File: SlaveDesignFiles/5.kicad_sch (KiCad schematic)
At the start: 43 parts, among them Q1 TXB0104PWR, Q2 TPS27082LDDCR, Q3 TPT75176B-SO1R, Q4 TPT75176B-SO1R

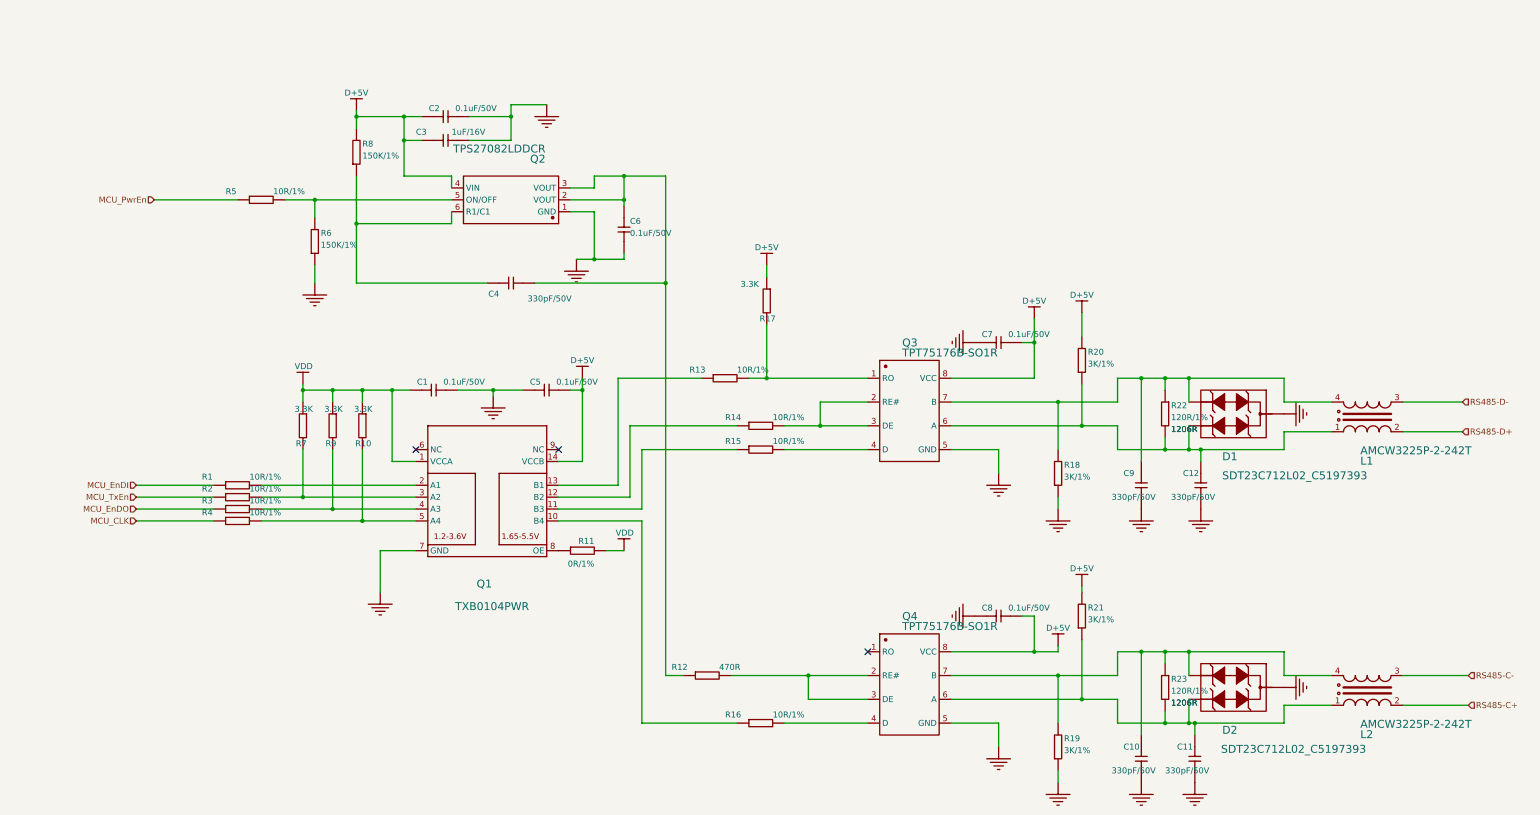
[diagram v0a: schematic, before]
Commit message: 28388d直接在底板上
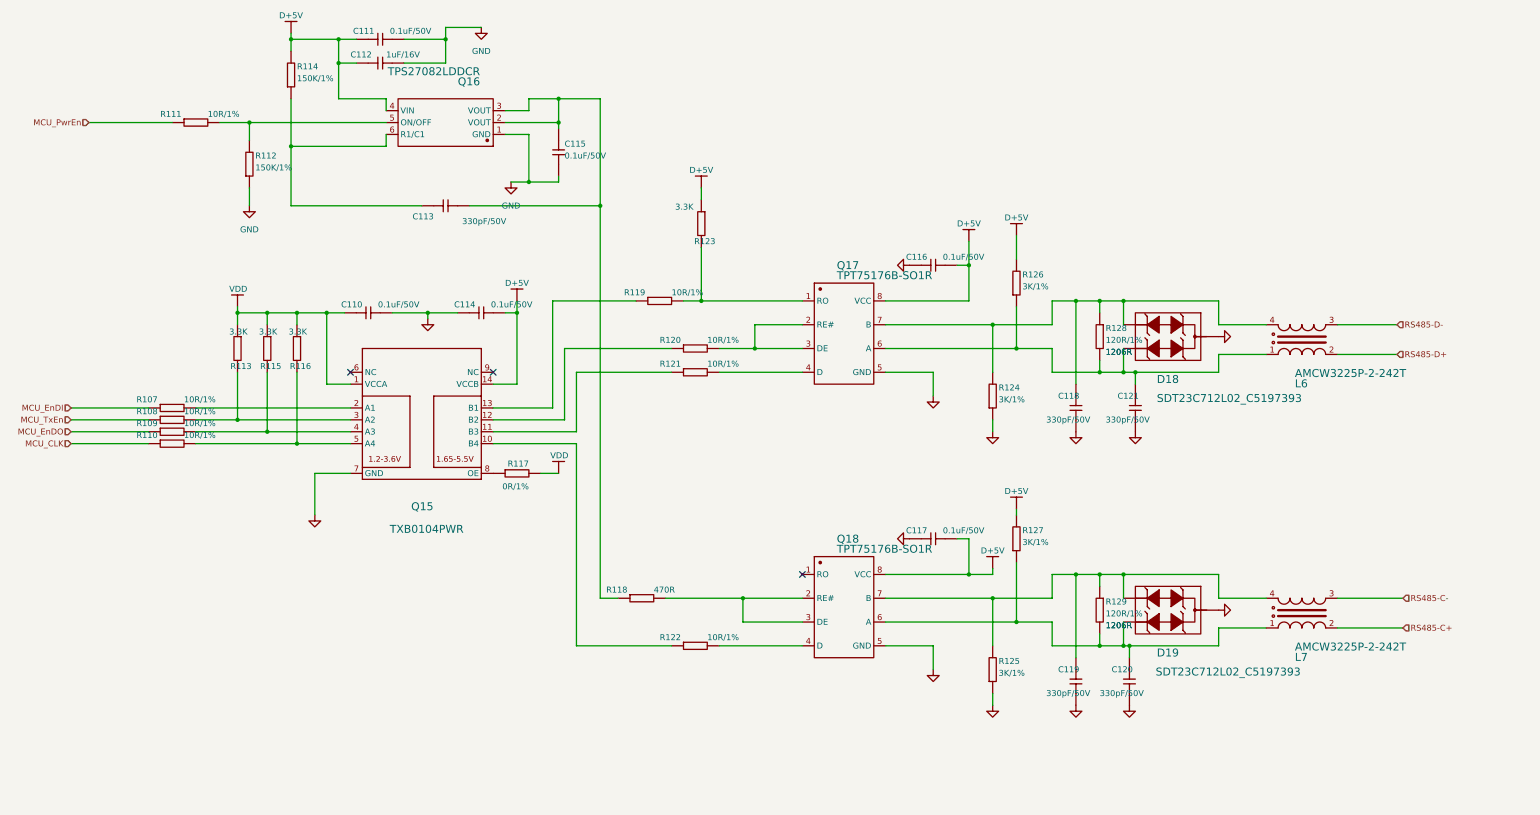
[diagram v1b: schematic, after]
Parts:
- removed C1, C2, C5, C6, C7, C8: 0.1uF/50V, Capacitor_SMD:C_0603_1608Metric, symbol sheet1-altium-import:CAP_2
- removed C10, C11, C12, C4, C9: 330pF/50V, Capacitor_SMD:C_0603_1608Metric, symbol sheet1-altium-import:CAP_1
- removed C3: 1uF/16V, Capacitor_SMD:C_0603_1608Metric, symbol sheet1-altium-import:CAP
- removed D1, D2: SDT23C712L02_C5197393, Lib2ic:SOT-23-3_L2.9-W1.3-P1.90-LS2.4-BR, symbol sheet1-altium-import:SDT23C712L02_C5197393
- removed L1, L2: AMCW3225P-2-242T, Lib_sheet_10:FILTER-SMD_4P-L3.2-W2.5-BL_WCM3225XXXX, symbol sheet1-altium-import:AMCW3225P-2-242T
- removed Q1: TXB0104PWR, Lib2ic:TSSOP-14_L5.0-W4.4-P0.65-LS6.4-BL, symbol sheet1-altium-import:TXB0104PWR
- removed Q2: TPS27082LDDCR, Lib_sheet_10:SOT-23-6_L2.9-W1.6-P0.95-LS2.8-BR, symbol sheet1-altium-import:TPS27082LDDCR
- removed Q3: TPT75176B-SO1R, Lib2ic:SOP-8_L4.9-W3.9-P1.27-LS6.0-BL, symbol sheet1-altium-import:TPT75176B-SO1R
- removed R1, R13, R14, R15, R16, R2, R3, R4, R5: 10R/1%, Resistor_SMD:R_0603_1608Metric, symbol sheet1-altium-import:RES_1
- removed R10, R17, R7, R9: 3.3K, Lib_sheet_10:R_0603_1608Metric, symbol sheet1-altium-import:RES_2
- removed R11: 0R/1%, Resistor_SMD:R_0603_1608Metric, symbol sheet1-altium-import:RES_7
- removed R12: 470R, Resistor_SMD:R_0603_1608Metric, symbol sheet1-altium-import:RES_6
- removed R18, R19, R20, R21: 3K/1%, Resistor_SMD:R_0603_1608Metric, symbol sheet1-altium-import:RES_3
- removed R22, R23: 120R/1%, Resistor_SMD:R_1206_3216Metric, symbol sheet1-altium-import:RES_5
- removed R6, R8: 150K/1%, Resistor_SMD:R_0603_1608Metric, symbol sheet1-altium-import:RES_4
- added C110, C111, C114, C115, C116, C117: 0.1uF/50V, Capacitor_SMD:C_0603_1608Metric, symbol sheet1-altium-import:CAP_2
- added C112: 1uF/16V, Capacitor_SMD:C_0603_1608Metric, symbol sheet1-altium-import:CAP
- added C113, C118, C119, C120, C121: 330pF/50V, Capacitor_SMD:C_0603_1608Metric, symbol sheet1-altium-import:CAP_1
- added D18, D19: SDT23C712L02_C5197393, Lib2ic:SOT-23-3_L2.9-W1.3-P1.90-LS2.4-BR, symbol sheet1-altium-import:SDT23C712L02_C5197393
- added L6, L7: AMCW3225P-2-242T, Lib_sheet_10:FILTER-SMD_4P-L3.2-W2.5-BL_WCM3225XXXX, symbol sheet1-altium-import:AMCW3225P-2-242T
- added Q15: TXB0104PWR, Lib2ic:TSSOP-14_L5.0-W4.4-P0.65-LS6.4-BL, symbol sheet1-altium-import:TXB0104PWR
- added Q16: TPS27082LDDCR, Lib_sheet_10:SOT-23-6_L2.9-W1.6-P0.95-LS2.8-BR, symbol sheet1-altium-import:TPS27082LDDCR
- added Q17: TPT75176B-SO1R, Lib2ic:SOP-8_L4.9-W3.9-P1.27-LS6.0-BL, symbol sheet1-altium-import:TPT75176B-SO1R
- added R107, R108, R109, R110, R111, R119, R120, R121, R122: 10R/1%, Resistor_SMD:R_0603_1608Metric, symbol sheet1-altium-import:RES_1
- added R112, R114: 150K/1%, Resistor_SMD:R_0603_1608Metric, symbol sheet1-altium-import:RES_4
- added R113, R115, R116, R123: 3.3K, Lib_sheet_10:R_0603_1608Metric, symbol sheet1-altium-import:RES_2
- added R117: 0R/1%, Resistor_SMD:R_0603_1608Metric, symbol sheet1-altium-import:RES_7
- added R118: 470R, Resistor_SMD:R_0603_1608Metric, symbol sheet1-altium-import:RES_6
- added R124, R125, R126, R127: 3K/1%, Resistor_SMD:R_0603_1608Metric, symbol sheet1-altium-import:RES_3
- added R128, R129: 120R/1%, Resistor_SMD:R_1206_3216Metric, symbol sheet1-altium-import:RES_5
- renumbered Q4 to Q18
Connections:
- net AGND: now also C110.2, C114.1, C116.1, C117.1, C118.2, C119.2, C120.2, C121.2, D18.3, D19.3, Q15.7 (GND), Q17.5 (GND), R124.1, R125.1
- net D+5V: now also C111.1, C112.1, C114.2, C116.2, C117.2, Q15.14 (VCCB), Q16.4 (VIN), Q17.8 (VCC), R114.2, R123.1, R126.2, R127.2
- net MCU_CLK: now also R110.1
- net MCU_EnDI: now also R107.1
- net MCU_EnDO: now also R109.1
- net MCU_PwrEn: now also R111.1
- net MCU_TxEn: now also R108.1
- net RS485-C+: now also L7.2
- net RS485-C-: now also L7.3
- net RS485-D+: now also L6.2
- net RS485-D-: now also L6.3
- net VDD: now also C110.1, Q15.1 (VCCA), R113.1, R115.1, R116.1, R117.2
- net at Q18.6 (A): now also C120.1, D19.2, L7.1, R127.1, R129.2
- net at Q18.7 (B): now also C119.1, D19.1, L7.4, R125.2, R129.1
- net at Q18.2 (RE#), Q18.3 (DE): now also R118.2
- net at Q18.4 (D): now also R122.2
- new net: C118.1, D18.1, L6.4, Q17.7 (B), R124.2, R128.1
- new net: C121.1, D18.2, L6.1, Q17.6 (A), R126.1, R128.2
- new net: Q15.8 (OE), R117.1
- new net: Q15.4 (A3), R109.2, R115.2
- new net: C113.2, C115.1, Q16.2 (VOUT), Q16.3 (VOUT), R118.1
- new net: Q16.5 (ON/OFF), R111.2, R112.2
- new net: C113.1, Q16.6 (R1/C1), R114.1
- new net: Q15.10 (B4), R122.1
- new net: Q15.2 (A1), R107.2
- new net: Q15.11 (B3), R121.1
- new net: Q15.12 (B2), R120.1
- new net: Q15.13 (B1), R119.1
- new net: Q15.3 (A2), R108.2, R113.2
- new net: Q15.5 (A4), R110.2, R116.2
- new net: Q17.1 (RO), R119.2, R123.2
- new net: Q17.2 (RE#), Q17.3 (DE), R120.2
- new net: Q17.4 (D), R121.2
- new net GND: C111.2, C112.2, C115.2, Q16.1 (GND), R112.1
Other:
- moved on the sheet: Q18
